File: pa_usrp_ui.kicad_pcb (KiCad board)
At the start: 4 copper layers, 59 x 39 mm, 18 parts, among them J1 BWSMA-KE-P001, J2 BWSMA-KE-P001, J3 2118722-2, U1 QPA9418TR13

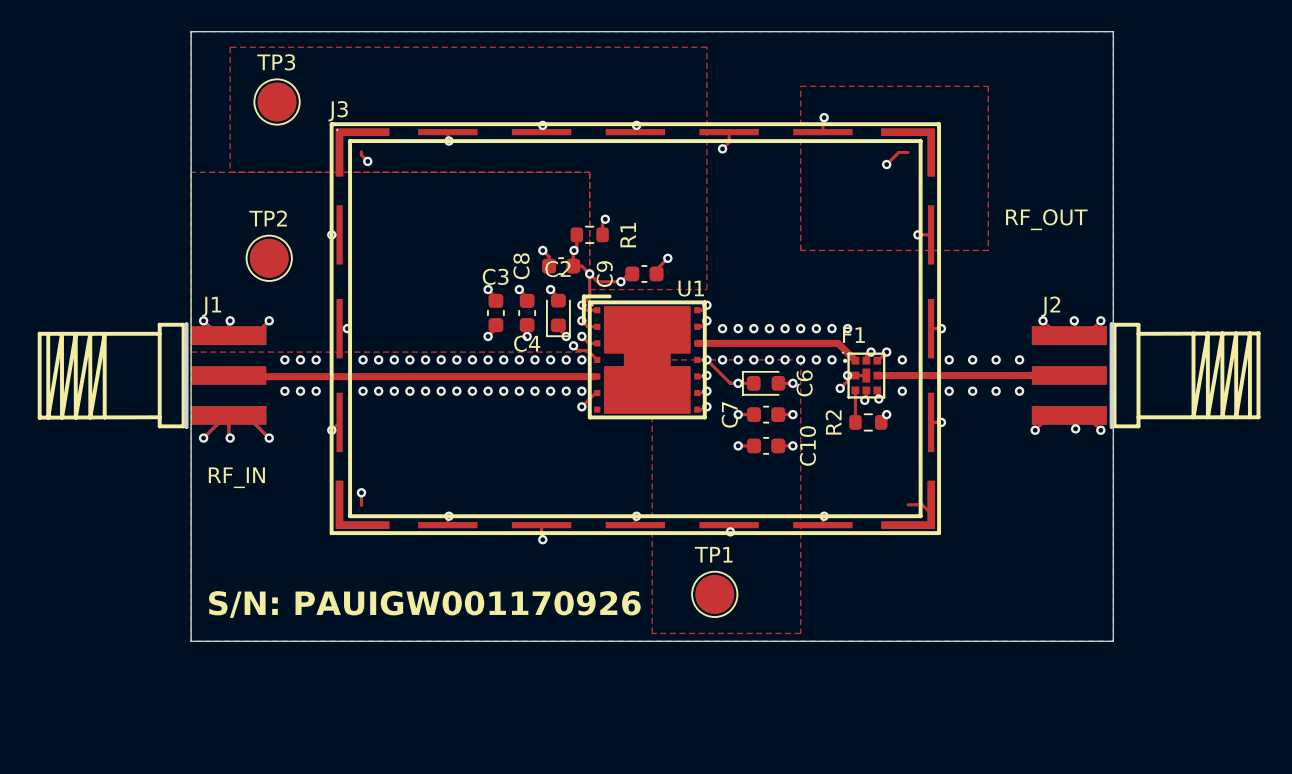
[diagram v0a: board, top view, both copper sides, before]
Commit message: Adding lna uplink
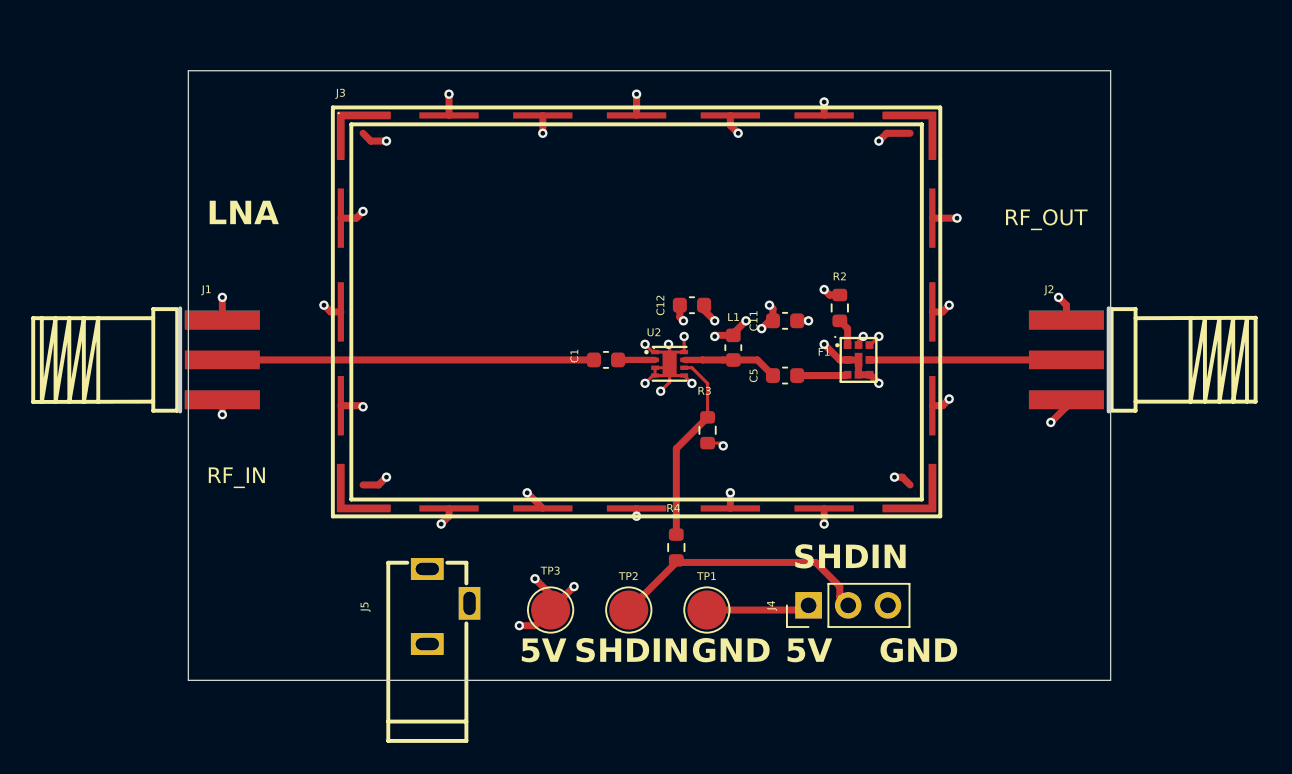
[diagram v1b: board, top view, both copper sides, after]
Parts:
- removed C10, C3, C9: 0.1uF, Capacitor_SMD:C_0603_1608Metric
- removed C2, C6: 10.0uF, Diode_SMD:D_0603_1608Metric
- removed C4, C7: 1000pF, Capacitor_SMD:C_0603_1608Metric
- removed C8: 100pF, Capacitor_SMD:C_0603_1608Metric
- removed R1: 0, Resistor_SMD:R_0603_1608Metric
- removed U1: QPA9418TR13, fooptrints:DFN-14_L7.0-W7.0-P1.06-TL-EP_QPA9418TR13
- added C1: 100pF, Capacitor_SMD:C_0603_1608Metric, F.Cu at (129.0, 89.5)
- added C11: 100pF, Capacitor_SMD:C_0603_1608Metric, F.Cu at (140.5, 87.0)
- added C12: 100pF, Capacitor_SMD:C_0603_1608Metric, F.Cu at (134.5, 86.0)
- added C5: 100pF, Capacitor_SMD:C_0603_1608Metric, F.Cu at (140.5, 90.5)
- added J4: Conn_01x03_Pin, Connector_PinHeader_2.54mm:PinHeader_1x03_P2.54mm_Vertical, F.Cu at (142.0, 105.2)
- added J5: HX DC002-1.3, fooptrints:DC-IN-TH_HANXIA_HX-DC002-1.3, F.Cu at (119.0, 105.3)
- added L1: 18nH, Inductor_SMD:L_0603_1608Metric, F.Cu at (137.2, 88.7)
- added R3: 10k, Resistor_SMD:R_0603_1608Metric, F.Cu at (135.5, 94.0)
- added R4: 33k, Resistor_SMD:R_0603_1608Metric, F.Cu at (133.5, 101.5)
- added U2: TQP3M9036, fooptrints:DFN-8_L2.0-W2.0-P0.50-BL-EP, F.Cu at (133.1, 89.8)
- TP1: value VCC1 -> GND
- TP2: value VCC2 -> SHDIN
- moved TP3 36.9 mm to (125.5, 105.5)
- moved TP2 32.2 mm to (130.5, 105.5), turned to 0 degrees
- moved R2 7.55 mm to (144.0, 86.2), turned to -90 degrees
- moved F1 1.12 mm to (145.2, 89.5)
- moved TP1 1.12 mm to (135.5, 105.5), turned to 0 degrees
- moved J1 1.08 mm to (104.5, 89.5)
- moved J3 1.07 mm to (131.0, 86.4)
- moved J2 1.02 mm to (158.5, 89.5)
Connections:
- R2 pad 2: Net-(F1-B3UL) -> Net-(F1-B3DL)
- TP1 pad 1: VCC2 -> GNDREF
- TP2 pad 1: VCC1 -> /SHDIN
- TP3 pad 1: VREF -> VDD
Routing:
- net /SHDIN: track 0.00 -> 16.8 mm
- net GNDREF: track 77.2 -> 61.5 mm, vias 117 -> 38
- net VDD: track 0.00 -> 12.4 mm, vias 0 -> 8
- net Net-(U2-Shutdown): track 0.00 -> 12.4 mm
- net Net-(U1-VREF): track 9.81 -> 0.00 mm, vias 4 -> 0
- net Net-(F1-B3DL): track 10.6 -> 1.76 mm
- net VCC2: track 6.26 -> 0.00 mm, vias 4 -> 0
- net Net-(U2-RFout): track 0.00 -> 6.10 mm
- net VCC1: track 4.47 -> 0.00 mm, vias 4 -> 0
- net Net-(U2-RFin): track 0.00 -> 2.37 mm
- net Net-(F1-B3UL): track 2.05 -> 3.25 mm
- net Net-(C1-Pad1): track 23.6 -> 22.4 mm
- net VREF: track 1.07 -> 0.00 mm, vias 1 -> 0
- added copper zone on In1.Cu, net GNDREF
- added copper zone on In2.Cu, net VDD
- removed copper zone on B.Cu, net GNDREF
- removed copper zone on F.Cu, net GNDREF
- removed copper zone on F.Cu, net VCC1
- removed copper zone on F.Cu, net VCC2
- removed copper zone on F.Cu, net VREF
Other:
- board text added: "5V"
- board text added: "GND"
- board text added: "LNA"
- board text added: "S/N: LNAIGW001170926"
- board text added: "SHDIN"
- board text removed: "S/N: PAUIGW001170926"
